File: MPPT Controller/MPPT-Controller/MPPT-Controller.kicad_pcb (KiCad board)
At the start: 4 copper layers, 79 parts, among them J1 Conn_01x02_Pin, J2 Conn_01x02_Pin, J3 Conn_01x02_Pin, J4 Conn_01x02_Pin, J5 USB_C_Receptacle_USB2.0_16P, J6 Conn_01x02_Pin, Q1 IRL540N, SW1 SW_SPDT, U1 ADS1115IDGS, U2 ESP32-WROOM-32D, U3 CH340C, U4 LM1117DT-3.3, U5 LM2596S-ADJ, U6 TC4422, U7 ADS1115IDGS

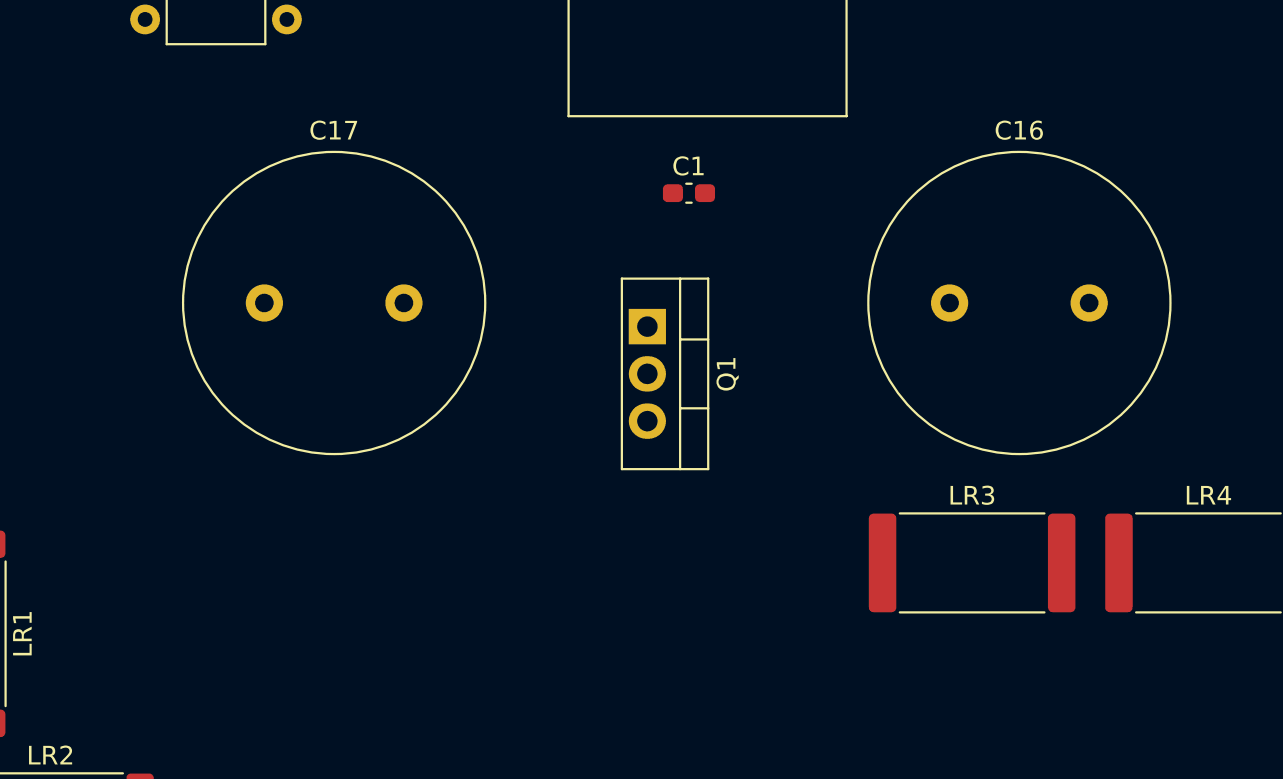
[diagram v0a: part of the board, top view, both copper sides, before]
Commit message: Capacitors
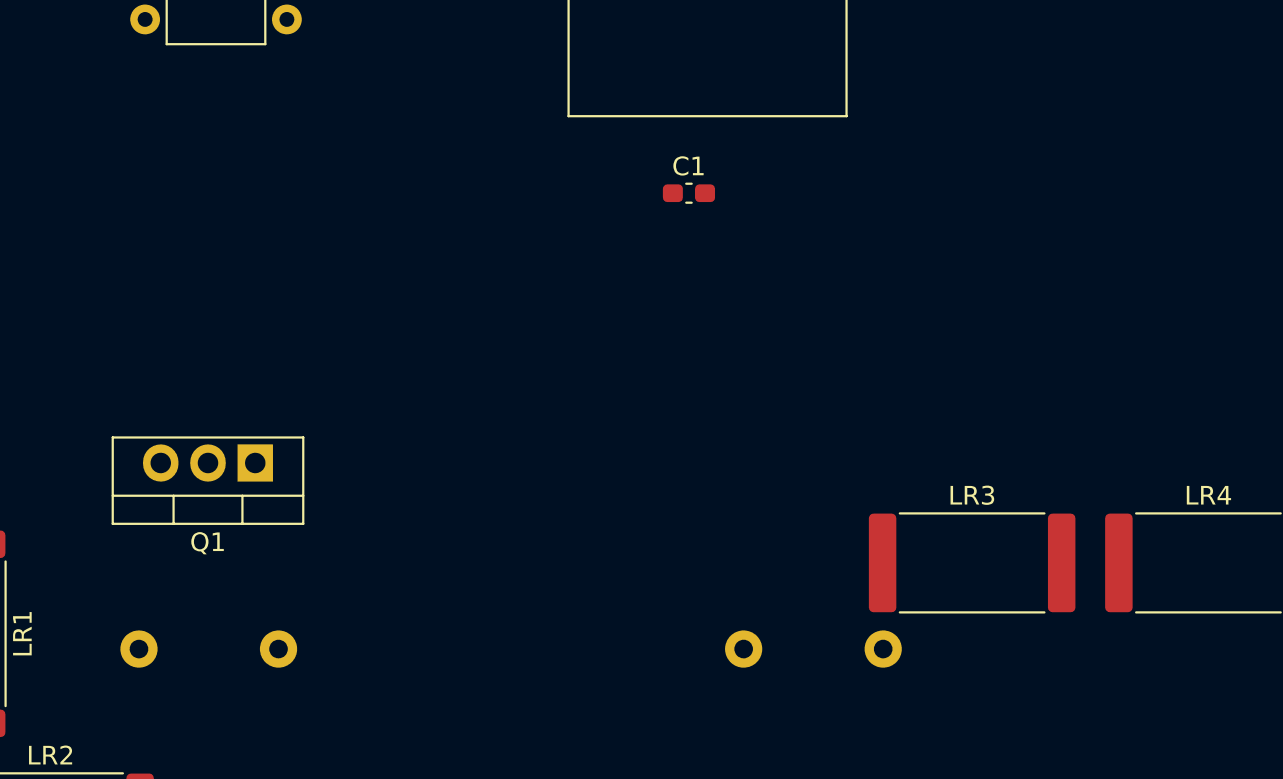
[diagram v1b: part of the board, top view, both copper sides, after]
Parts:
- C16, C17: moved to B.Cu
- moved Q1 22.3 mm to (74.5, 97.5), turned to 180 degrees
- moved C17 19.8 mm to (68.2, 107.5)
- moved C16 18.9 mm to (108.2, 107.5), turned to 180 degrees
